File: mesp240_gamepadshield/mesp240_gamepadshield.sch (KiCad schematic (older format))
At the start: 30 parts, among them J1 1.27P CNX, J2 1.27P CNX, J3 Piezo Connector, Q1 MMBT3904, SW1 Button DOWN, SW2 Button LEFT, SW3 Button Right, SW4 Button UP, SW5 Button B, SW6 Button X, SW7 Button Y, SW8 Button A

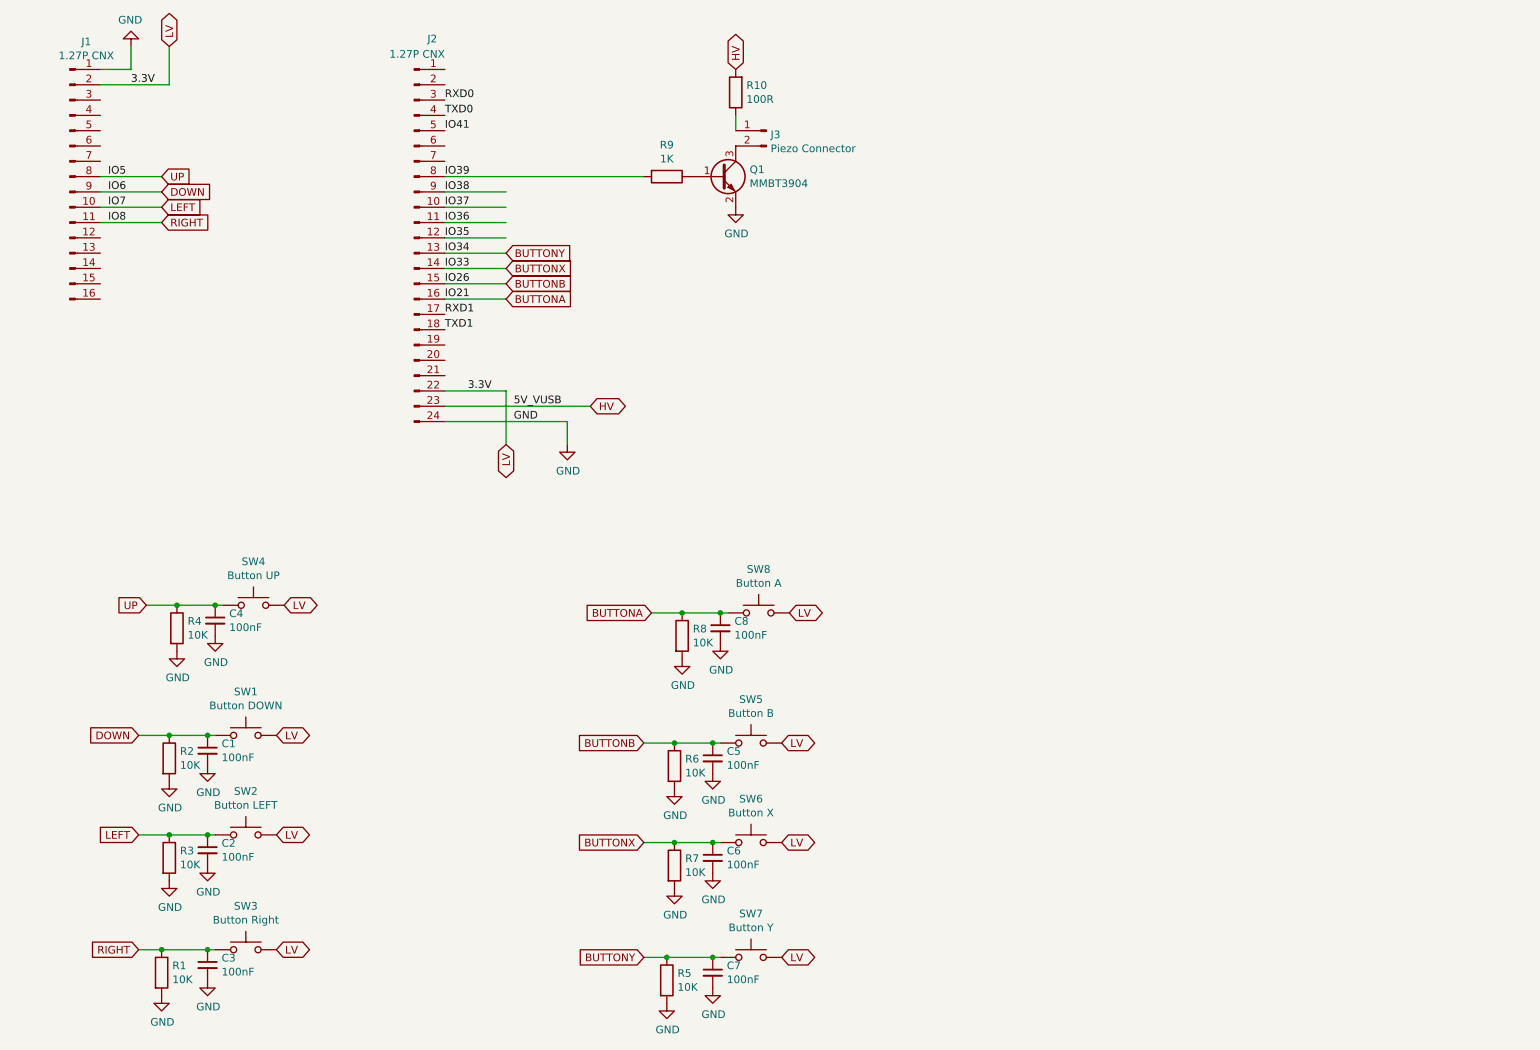
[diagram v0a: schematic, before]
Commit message: updated Schematic + pdf
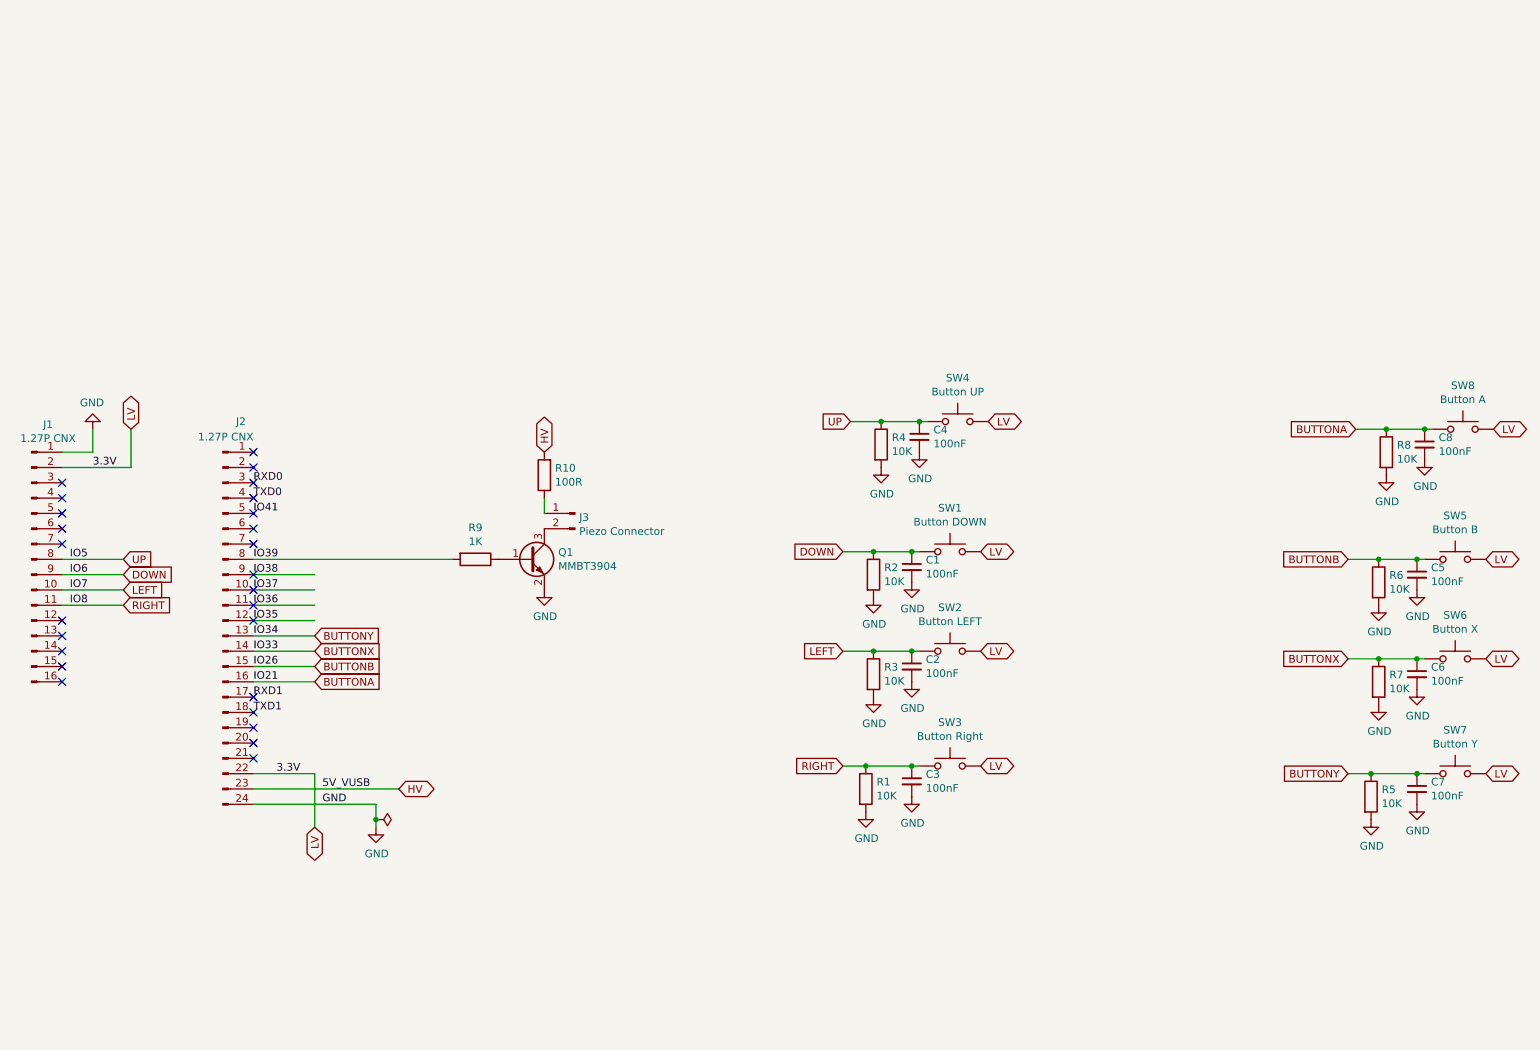
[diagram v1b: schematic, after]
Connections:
- wire segments 47 -> 48
- no-connect marks 0 -> 26
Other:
- moved on the sheet: C1, C2, C3, C4, C5, C6, C7, C8, J1, J2, J3, Q1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
